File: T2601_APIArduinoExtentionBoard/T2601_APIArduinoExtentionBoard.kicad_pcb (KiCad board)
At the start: 2 copper layers, 60 x 90 mm, 90 parts, among them J1 Conn_01x10_Socket, J11 Conn_01x04_Pin, J12 Screw_Terminal_01x02, J13 Conn_01x04_Pin, J14 Screw_Terminal_01x02, J15 Conn_02x08_Counter_Clockwise, J2 Conn_01x10_Socket, J3 Conn_01x10_Socket, J4 Conn_01x10_Socket, J5 Screw_Terminal_01x08, J6 Screw_Terminal_01x08, J7 Conn_02x03_Counter_Clockwise, J8 Conn_01x04, J9 Conn_02x08_Counter_Clockwise, U1 ATMEGA328P-AU, X1 X322516MOB4SI

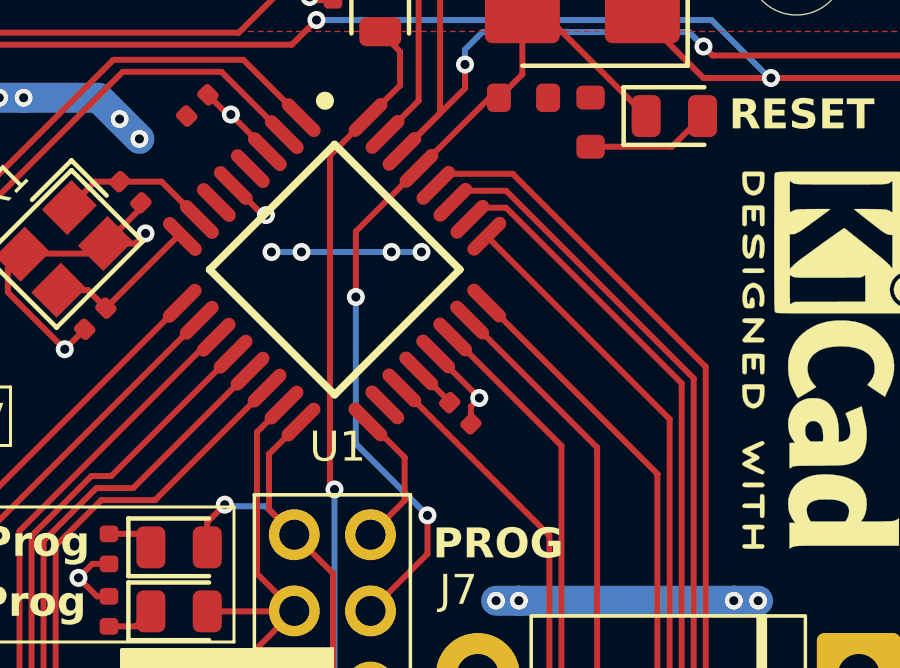
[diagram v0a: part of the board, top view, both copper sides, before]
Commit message: 3D models
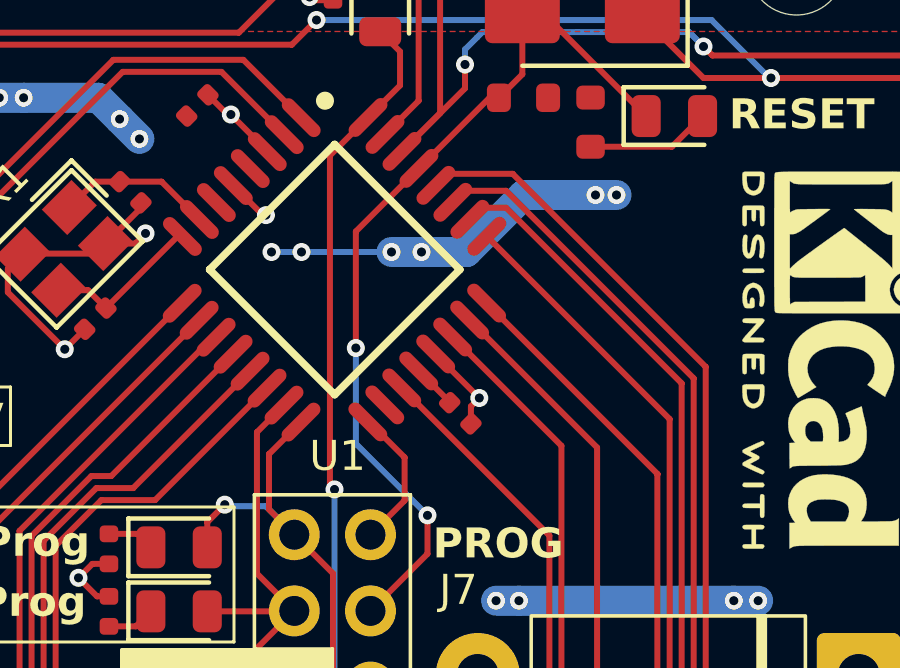
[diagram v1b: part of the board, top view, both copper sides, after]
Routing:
- net +5V: track 60.7 -> 68.0 mm, vias 22 -> 24
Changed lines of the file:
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@@
 		(at 155.6004 57.092435 -135)
 		(property "Reference" "U1"
-			(at 4.09978 -4.243464 0)
+			(at 4.318983 -4.459839 0)
 			(layer "F.SilkS")
 			(effects
@@
 		)
 		(embedded_fonts no)
-		(model "${EASYEDA2KICAD}/easyeda2kicad.3dshapes/TQFP-32_L7.0-W7.0-H1.2-LS9.0-P0.80.wrl"
+		(model "${KIPRJMOD}/M2601_APIArduinoExtentionBoard_Lib3D/TQFP-32_L7.0-W7.0-H1.2-LS9.0-P0.80.wrl"
 			(offset
 				(xyz -0 0 -0)
@@
 		)
 		(embedded_fonts no)
-		(model "${EASYEDA2KICAD}/easyeda2kicad.3dshapes/CRYSTAL-SMD_4P-L3.2-W2.5-BL.wrl"
+		(model "${KIPRJMOD}/M2601_APIArduinoExtentionBoard_Lib3D/CRYSTAL-SMD_4P-L3.2-W2.5-BL.step"
 			(offset
 				(xyz 0 -0 -0)
@@
 	)
 	(via
+		(at 164.3 54.6)
+		(size 0.6)
+		(drill 0.3)
+		(layers "F.Cu" "B.Cu")
+		(net 4)
+	)
+	(via
 		(at 137.94 51.42)
 		(size 0.6)
@@
 	)
 	(via
+		(at 165 54.6)
+		(size 0.6)
+		(drill 0.3)
+		(layers "F.Cu" "B.Cu")
+		(net 4)
+	)
+	(via
 		(at 168.91 68.1228)
 		(size 0.6)
@@
 	)
 	(segment
+		(start 164.3 54.6)
+		(end 165 54.6)
+		(width 1)
+		(layer "B.Cu")
+		(net 4)
+	)
+	(segment
+		(start 160 56.5)
+		(end 161.9 54.6)
+		(width 1)
+		(layer "B.Cu")
+		(net 4)
+	)
+	(segment
 		(start 144.4244 51.3588)
 		(end 145.2372 51.3588)
@@
 	)
 	(segment
+		(start 158.5 56.5)
+		(end 160 56.5)
+		(width 1)
+		(layer "B.Cu")
+		(net 4)
+	)
+	(segment
+		(start 161.9 54.6)
+		(end 164.3 54.6)
+		(width 1)
+		(layer "B.Cu")
+		(net 4)
+	)
+	(segment
 		(start 173.0756 70.7136)
 		(end 173.0756 70.6)
@@
 	)
 	(segment
-		(start 158.5 56.5)
-		(end 153.5 56.5)
+		(start 154.5 56.5)
+		(end 157.5 56.5)
 		(width 0.2)
 		(layer "B.Cu")
@@
 	)
 	(segment
+		(start 158.5 56.5)
+		(end 157.5 56.5)
+		(width 1)
+		(layer "B.Cu")
+		(net 4)
+	)
+	(segment
 		(start 170.434 77.724)
 		(end 170.434 73.3552)
@@
 	)
 	(segment
+		(start 153.5 56.5)
+		(end 154.5 56.5)
+		(width 0.2)
+		(layer "B.Cu")
+		(net 4)
+	)
+	(segment
 		(start 149.098 52.7304)
 		(end 148.4376 52.07)
@@
 	)
 	(segment
+		(start 156.3116 59.7)
+		(end 156.3116 55.81555)
+		(width 0.2)
+		(layer "F.Cu")
+		(net 28)
+	)
+	(segment
 		(start 161.861999 50.5764)
 		(end 161.079599 51.3588)
@@
 	)
 	(segment
+		(start 156.3116 55.81555)
+		(end 158.414685 53.712465)
+		(width 0.2)
+		(layer "F.Cu")
+		(net 28)
+	)
+	(segment
 		(start 161.861999 48.641)
 		(end 161.7 48.479001)
@@
 	)
 	(segment
-		(start 156.3116 58)
-		(end 156.3116 55.81555)
-		(width 0.2)
-		(layer "F.Cu")
-		(net 28)
-	)
-	(segment
 		(start 161.861999 48.641)
 		(end 162.6614 48.641)
@@
 	)
 	(segment
-		(start 156.3116 55.81555)
-		(end 158.414685 53.712465)
-		(width 0.2)
-		(layer "F.Cu")
-		(net 28)
-	)
-	(segment
 		(start 162.6614 48.641)
 		(end 165.9888 51.9684)
@@
 	)
 	(via
-		(at 156.3116 58)
+		(at 156.3116 59.7)
 		(size 0.6)
 		(drill 0.3)
@@
 	)
 	(segment
-		(start 156.3116 58)
+		(start 156.3116 59.7)
 		(end 156.3116 62.8904)
 		(width 0.2)
